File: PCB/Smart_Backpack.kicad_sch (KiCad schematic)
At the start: 24 parts, among them SW1 SW_Push, SW2 SW_Push, U3 ESP32-PICO-MINI-02-N8R2, U4 CP2102N-Axx-xQFN28

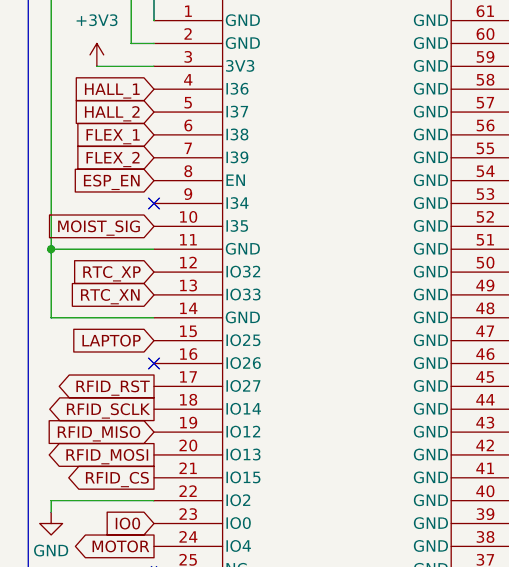
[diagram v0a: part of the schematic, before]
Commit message: This time for sure...
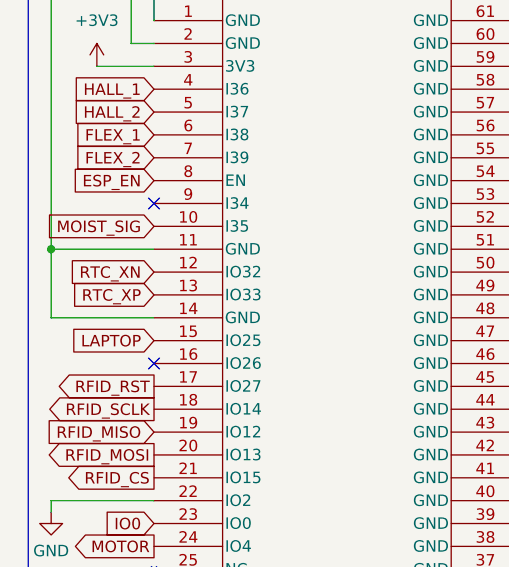
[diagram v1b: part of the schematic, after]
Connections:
- net RTC_XN: now also U3.12 (IO32); no longer U3.13 (IO33)
- net RTC_XP: now also U3.13 (IO33); no longer U3.12 (IO32)
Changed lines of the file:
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@@
 	(global_label "RTC_XP"
 		(shape input)
-		(at 27.94 63.5 180)
-		(fields_autoplaced yes)
-		(effects
-			(font
-				(size 1.27 1.27)
-			)
-			(justify right)
-		)
-		(property "Intersheetrefs" "${INTERSHEET_REFS}"
-			(at 18.0001 63.5 0)
+		(at 27.94 66.04 180)
+		(fields_autoplaced yes)
+		(effects
+			(font
+				(size 1.27 1.27)
+			)
+			(justify right)
+		)
+		(property "Intersheetrefs" "${INTERSHEET_REFS}"
+			(at 17.9396 66.04 0)
 			(effects
 				(font
@@
 	(global_label "RTC_XN"
 		(shape input)
-		(at 27.94 66.04 180)
-		(fields_autoplaced yes)
-		(effects
-			(font
-				(size 1.27 1.27)
-			)
-			(justify right)
-		)
-		(property "Intersheetrefs" "${INTERSHEET_REFS}"
-			(at 17.9396 66.04 0)
-			(effects
-				(font
+		(at 27.94 63.5 180)
+		(fields_autoplaced yes)
+		(effects
+			(font
+				(size 1.27 1.27)
+			)
+			(justify right)
+		)
+		(property "Intersheetrefs" "${INTERSHEET_REFS}"
+			(at 18.0001 63.5 0)
+			(effects
+				(font
